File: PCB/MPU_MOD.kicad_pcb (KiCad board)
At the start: 8 copper layers, 45 x 70 mm, 305 parts, among them J1 SJ3-35024K-SMT-TR, J2 2-1734248-0, J501 MEM2090-00-145-00-A_REVA, J701 FTSH-107-01-L-DV-K-A, J801 USB4215-03-A_REVA, J901 73412-0110, U1 IS21ES08GA-JQLI-TR, U201 STC3115IQT, U203 STPMIC1APQR, U3 BQ24298RTWR, U301 STM32MP157FABx, U401 MT41K256M16TW-107_P, U502 HSP051-4M10, U503 HSP051-4M10, U701 HSP051-4M10, U702 HSP051-4M10, U801 FUSB302BMPX, U802 HSP051-4M10, U901 LBEE5PK2AE-771, Y601 NX2012SA-32.768K, Y701 ECS-2520MVQ-240

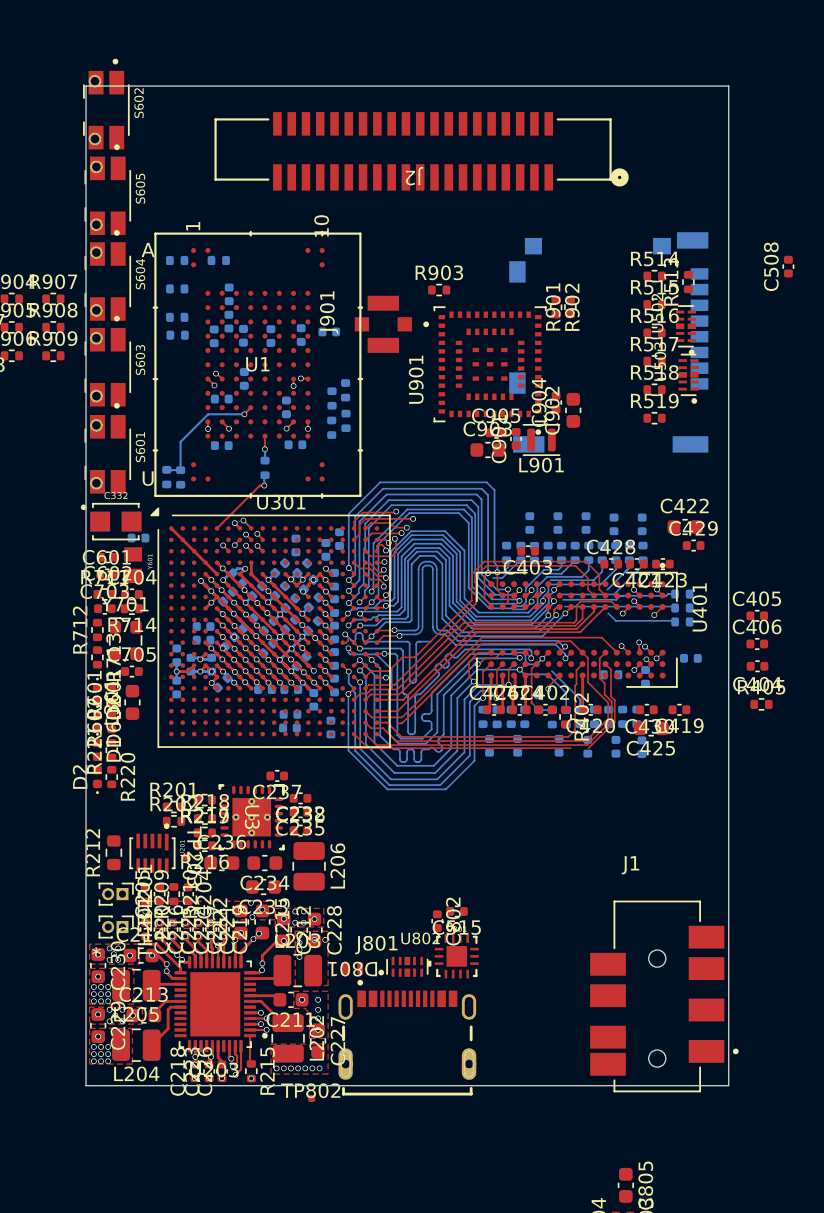
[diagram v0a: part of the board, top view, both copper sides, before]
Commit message: PCD_UPDATE
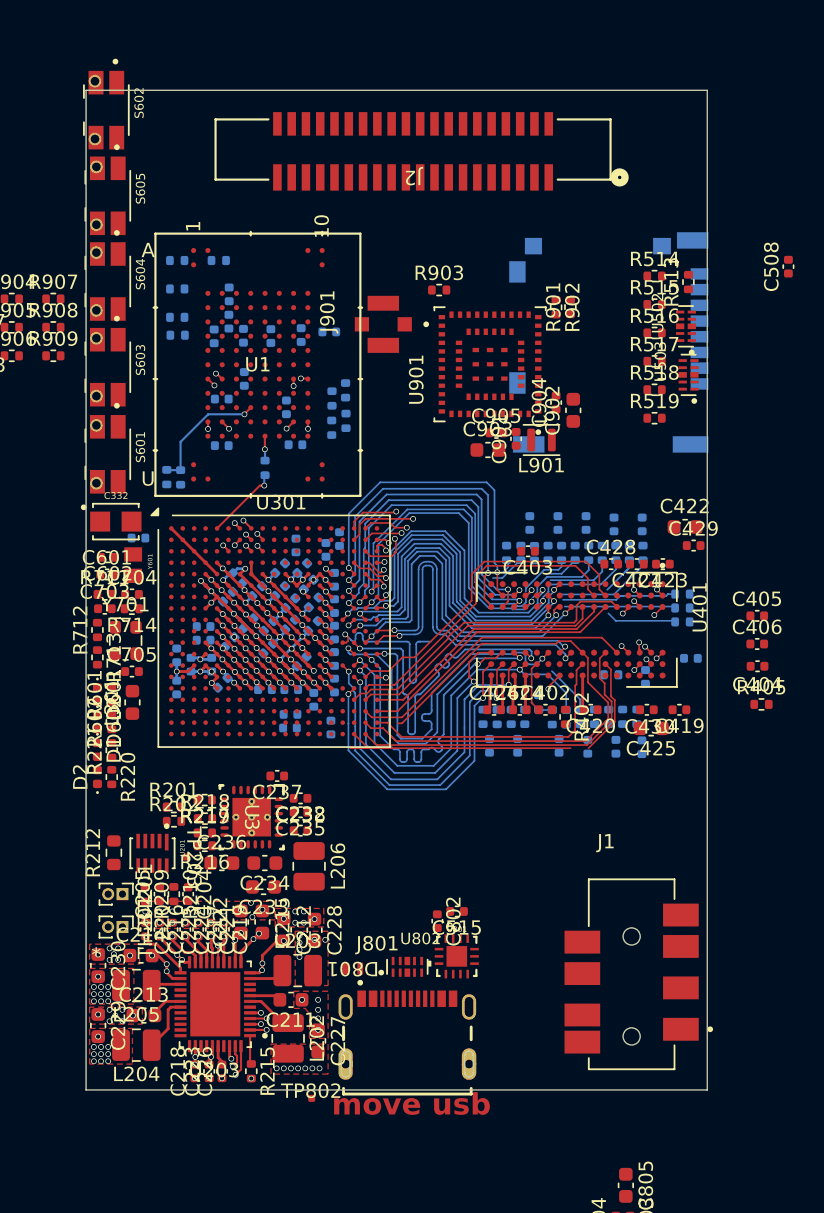
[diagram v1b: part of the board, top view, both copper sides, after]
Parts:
- moved J1 2.37 mm to (110.2, 96.8)
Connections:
- U401 pad H7: /DDR/DDR_DQ14 -> /DDR/DDR_DQ11
- U401 pad H8: /DDR/DDR_DQ11 -> /DDR/DDR_DQ14
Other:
- board size 45 x 70 mm -> 43.5 x 70 mm
- board text added: "move usb"
